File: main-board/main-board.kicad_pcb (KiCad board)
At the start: 2 copper layers, 99.8 x 66.8 mm, 41 parts, among them J1 Conn_02x08_Odd_Even, J2 Bat, Q1 AO3400A, Q2 AO3400A, Q3 AO3400A, Q4 AO3400A, Q5 AO3400A, Q6 AO3400A, Q7 AO3400A, Q8 AO3400A, U1 40106, U2 4024, U3 4040, U4 27C256, U5 LM78L05, U6 ULN2803A, U7 4028

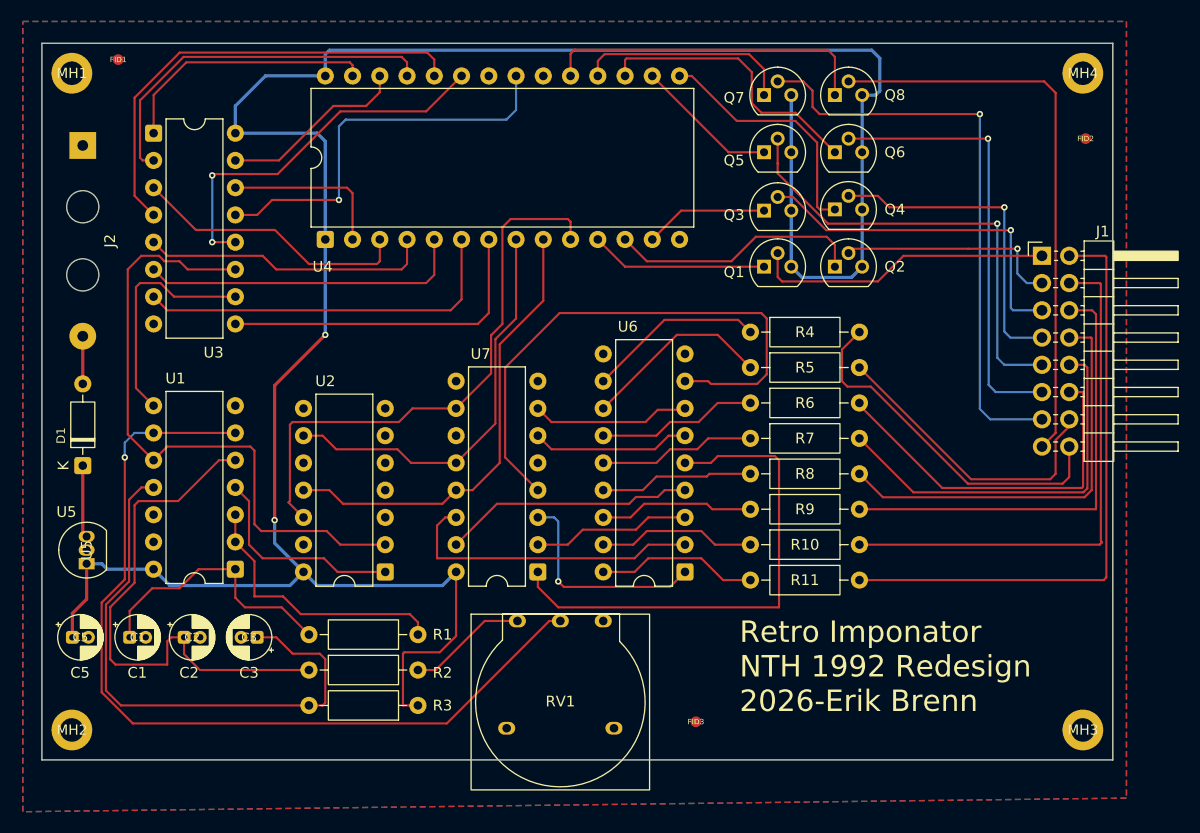
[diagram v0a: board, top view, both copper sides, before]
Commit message: Finalized Rev-1.0
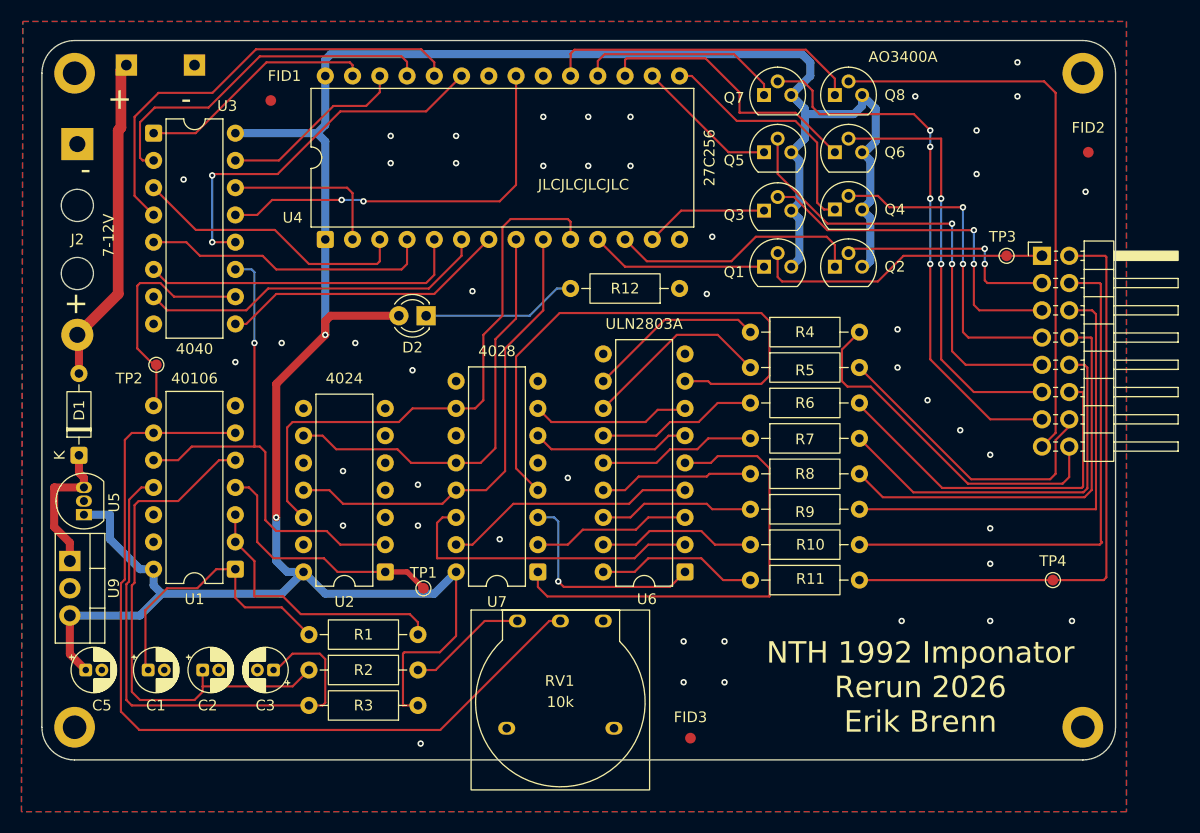
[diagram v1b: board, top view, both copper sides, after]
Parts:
- added D2: LED, LED_THT:LED_D3.0mm, F.Cu at (135.4, 83.3)
- added R12: 360, Resistor_THT:R_Axial_DIN0207_L6.3mm_D2.5mm_P10.16mm_Horizontal, F.Cu at (159.0, 80.8)
- added TP1: TestPoint, ezee-footprints:TestPoint_Pad_D1.0mm, F.Cu at (135.1, 108.7)
- added TP2: TestPoint, ezee-footprints:TestPoint_Pad_D1.0mm, F.Cu at (110.2, 87.9)
- added TP3: TestPoint, ezee-footprints:TestPoint_Pad_D1.0mm, F.Cu at (189.5, 77.7)
- added TP4: TestPoint, ezee-footprints:TestPoint_Pad_D1.0mm, F.Cu at (193.8, 108.0)
- added TPH1: TestPoint_Hook, ezee-footprints:TestPoint_Hook, F.Cu at (107.4, 59.9)
- added TPH2: TestPoint_Hook, ezee-footprints:TestPoint_Hook, F.Cu at (113.8, 59.9)
- added U9: L7805, Package_TO_SOT_THT:TO-220-3_Vertical, F.Cu at (102.2, 106.2)
- J2: value Bat -> 7-12V
- moved FID1 14.7 mm to (120.9, 63.2)
- moved U5 4.58 mm to (103.5, 101.9)
- moved C1 3.50 mm to (109.5, 116.3)
- moved C2 3.50 mm to (114.6, 116.3)
- moved C3 3.41 mm to (121.2, 116.3)
- moved C5 3.29 mm to (103.7, 116.3)
- moved FID3 1.61 mm to (160.0, 122.7)
- moved FID2 1.30 mm to (197.1, 68.1)
- moved D1 1.03 mm to (103.0, 96.3)
- moved J2 0.52 mm to (102.9, 85.1)
- moved MH2 0.36 mm to (102.6, 121.7)
- moved MH1 0.25 mm to (102.6, 60.7)
- moved MH3 0.25 mm to (196.6, 121.7)
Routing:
- net Net-(D1-A): track 4.45 -> 31.4 mm
- net Net-(D2-K): track 0.00 -> 14.5 mm
- net +5V: track 224.5 -> 236.7 mm
- net Net-(U2-MR): track 59.8 -> 47.8 mm, vias 0 -> 1
- net Net-(D1-K): track 6.75 -> 14.1 mm
- net Net-(U2-~{CLK}): track 19.6 -> 24.0 mm
- net Net-(U3-Q0): track 30.9 -> 26.9 mm
- net Net-(C3-Pad1): track 53.8 -> 50.1 mm
- net Net-(U6-I5): track 47.6 -> 43.9 mm
- net Net-(J1-Pin_13): track 54.7 -> 51.1 mm, vias 1 -> 4
- net Net-(U3-Q1): track 35.2 -> 32.9 mm
- net Net-(U3-Q11): track 24.5 -> 22.4 mm
- net Net-(C1-Pad1): track 24.9 -> 26.6 mm
- net Net-(J1-Pin_11): track 41.3 -> 39.9 mm, vias 1 -> 2
- net Net-(U2-Q2): track 38.4 -> 39.8 mm
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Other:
- board size 99.8 x 66.8 mm -> 100.1 x 67.1 mm
- board text added: "+"
- board text added: "-"
- board text added: "JLCJLCJLCJLC"
- board text added: "NTH 1992 Imponator Rerun 2026 Erik Brenn"
- board text removed: "Retro Imponator NTH 1992 Redesign 2026-Erik Brenn"
